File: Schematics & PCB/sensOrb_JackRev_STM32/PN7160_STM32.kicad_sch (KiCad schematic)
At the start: 3 parts, among them J1 USB_C_Receptacle_USB2.0_16P, U1 PN7160A1HN/C100E, U2 STM32F411CEUx

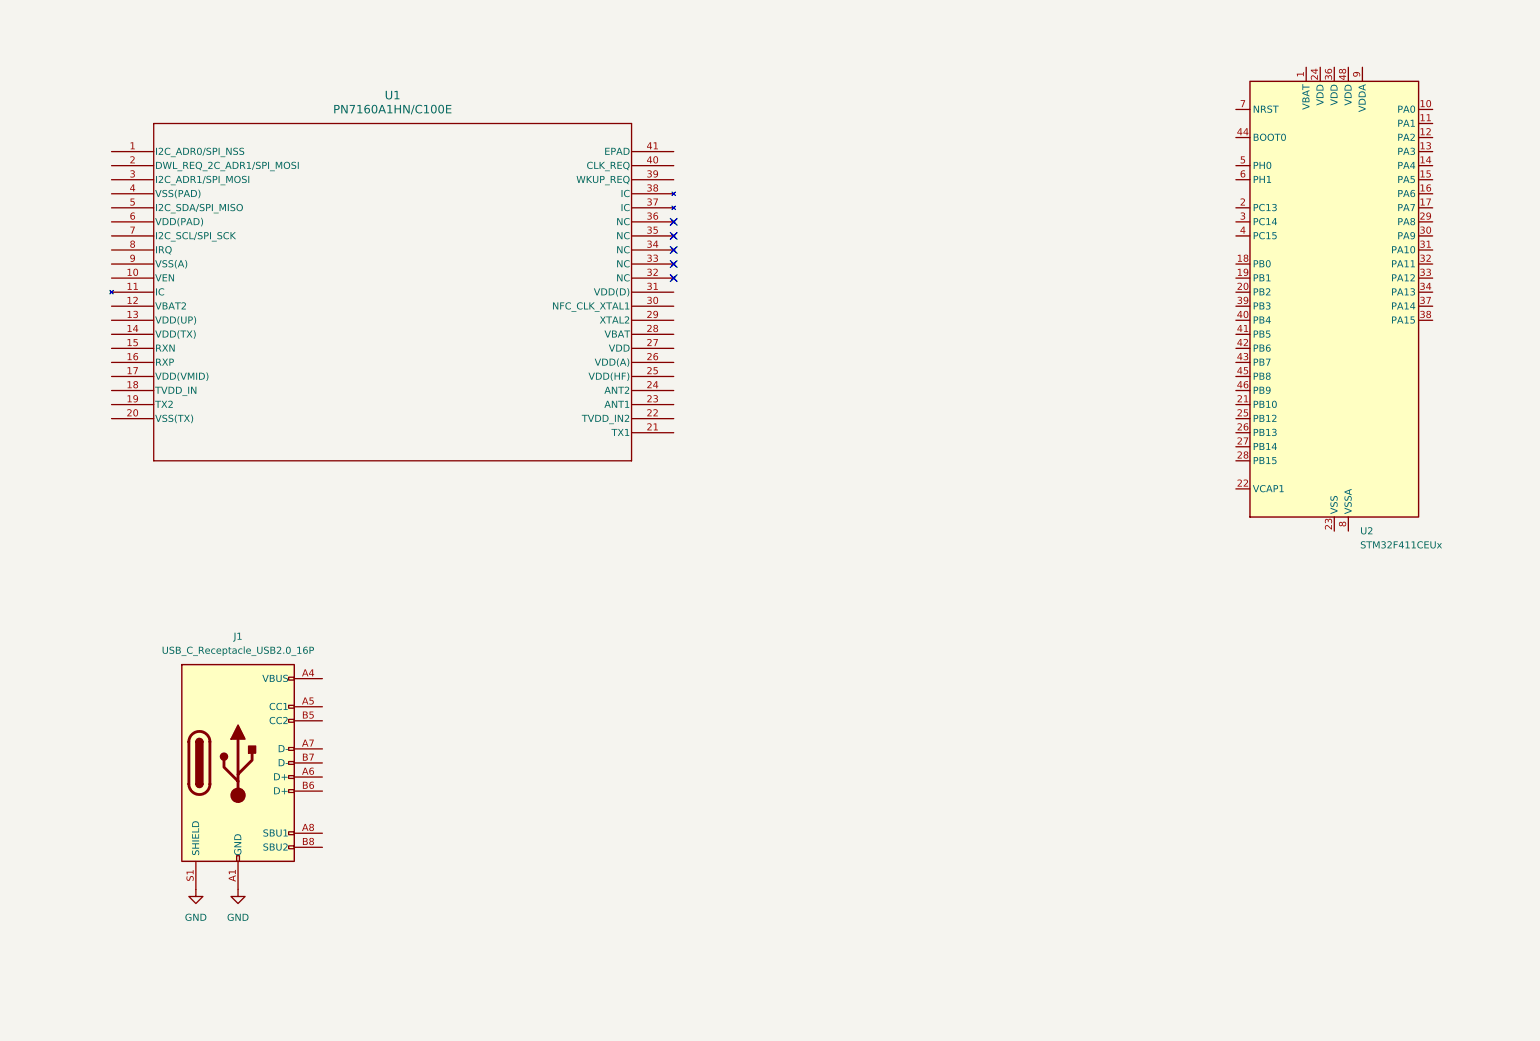
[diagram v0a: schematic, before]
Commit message: Baro unit design complete, core unit nearly done
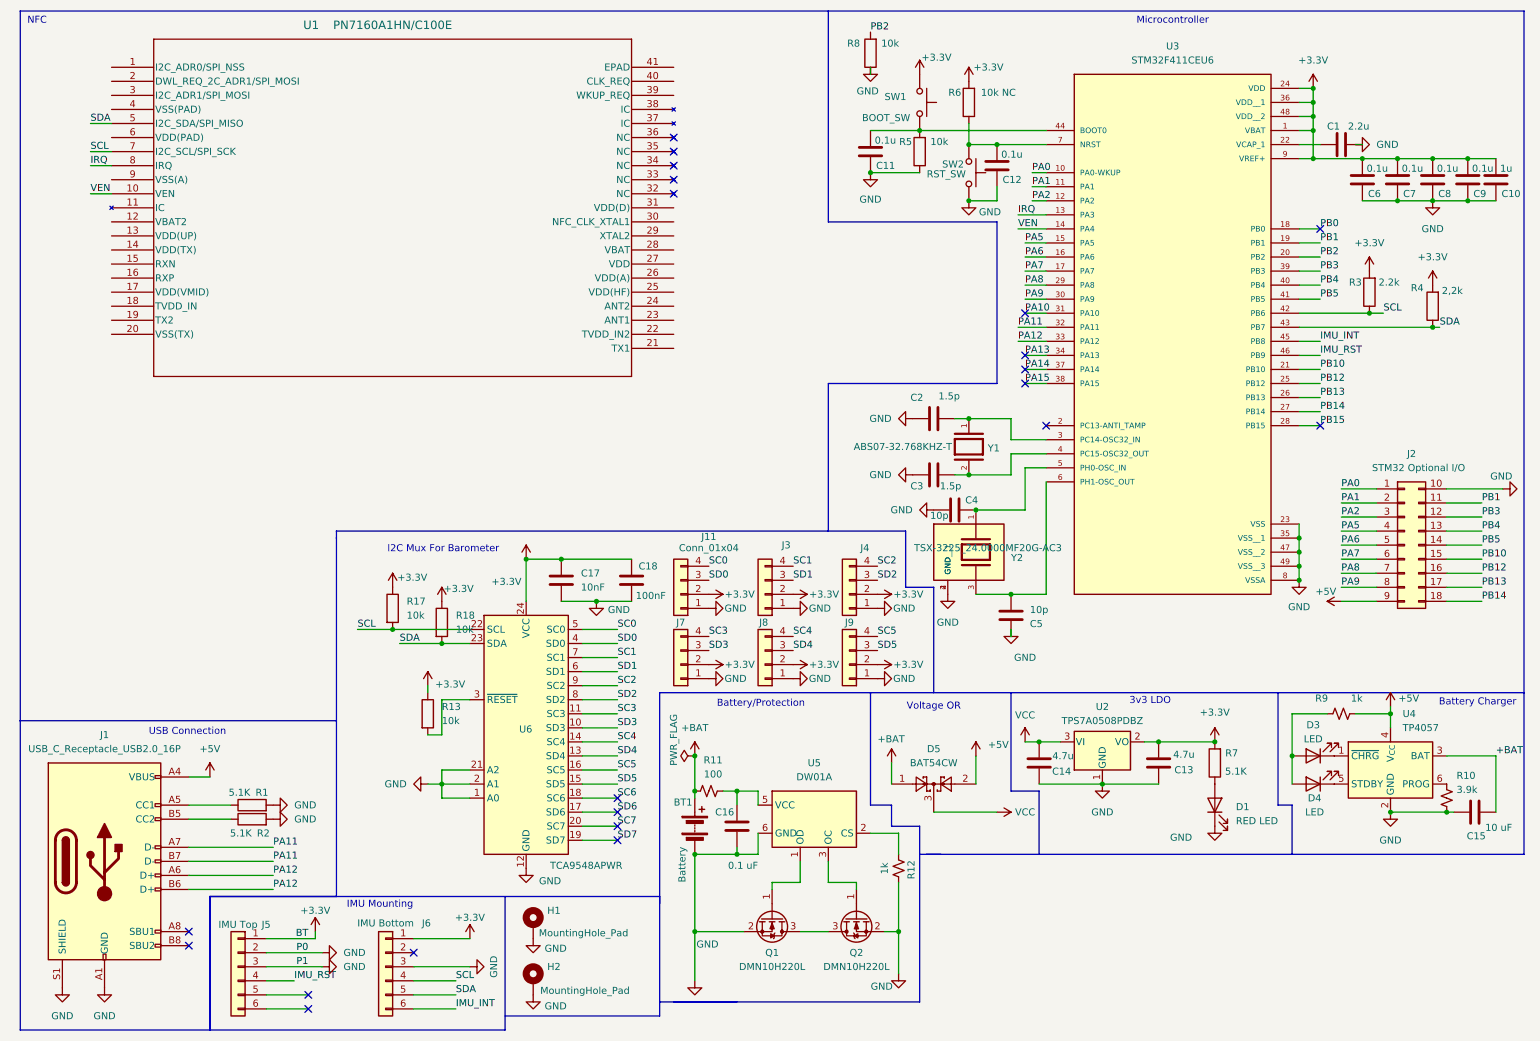
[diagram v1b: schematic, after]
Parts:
- removed U2: STM32F411CEUx, Package_DFN_QFN:QFN-48-1EP_7x7mm_P0.5mm_EP5.6x5.6mm, symbol MCU_ST_STM32F4:STM32F411CEUx
- added BT1: Battery, Battery:BatteryHolder_Keystone_1060_1x2032, symbol Device:Battery
- added C1: 2.2u, symbol Device:C
- added C10: 1u, symbol Device:C
- added C11, C12, C6, C7, C8, C9: 0.1u, symbol Device:C
- added C13, C14: 4.7u, symbol Device:C
- added C15: 10 uF, Capacitor_SMD:C_0805_2012Metric_Pad1.18x1.45mm_HandSolder, symbol Device:C
- added C16: 0.1 uF, Capacitor_SMD:C_0805_2012Metric_Pad1.18x1.45mm_HandSolder, symbol Device:C
- added C17: 10nF, Capacitor_SMD:C_0805_2012Metric_Pad1.18x1.45mm_HandSolder, symbol Device:C
- added C18: 100nF, Capacitor_SMD:C_0805_2012Metric_Pad1.18x1.45mm_HandSolder, symbol Device:C
- added C2, C3: 1.5p, symbol Device:C
- added C4, C5: 10p, symbol Device:C
- added D1: RED LED, symbol Device:LED
- added D3, D4: LED, LED_SMD:LED_0805_2012Metric, symbol Device:LED
- added D5: BAT54CW, Package_TO_SOT_SMD:SOT-323_SC-70, symbol Diode:BAT54CW
- added H1, H2: MountingHole_Pad, MountingHole:MountingHole_2.2mm_M2_Pad, symbol Mechanical:MountingHole_Pad
- added J11, J3, J4, J7, J8, J9: Conn_01x04, Connector_JST:JST_XH_B4B-XH-AM_1x04_P2.50mm_Vertical, symbol Connector_Generic:Conn_01x04
- added J2: STM32 Optional I/O, Connector_PinSocket_2.54mm:PinSocket_2x09_P2.54mm_Vertical, symbol Connector_Generic:Conn_02x09_Top_Bottom
- added J5: IMU Top, Connector_PinSocket_2.54mm:PinSocket_1x06_P2.54mm_Vertical, symbol Connector_Generic:Conn_01x06
- added J6: IMU Bottom, Connector_PinSocket_2.54mm:PinSocket_1x06_P2.54mm_Vertical, symbol Connector_Generic:Conn_01x06
- added Q1, Q2: DMN10H220L, Package_TO_SOT_SMD:SOT-23, symbol Transistor_FET:DMN10H220L
- added R1, R2, R7: 5.1K, symbol Device:R
- added R10: 3.9k, Resistor_SMD:R_0805_2012Metric_Pad1.20x1.40mm_HandSolder, symbol Device:R_Small_US
- added R11: 100, Resistor_SMD:R_0805_2012Metric_Pad1.20x1.40mm_HandSolder, symbol Device:R_Small_US
- added R12, R9: 1k, Resistor_SMD:R_0805_2012Metric_Pad1.20x1.40mm_HandSolder, symbol Device:R_Small_US
- added R13, R17, R18: 10k, Resistor_SMD:R_0805_2012Metric_Pad1.20x1.40mm_HandSolder, symbol Device:R
- added R3: 2.2k, symbol Device:R
- added R4: 2,2k, symbol Device:R
- added R5, R8: 10k, symbol Device:R
- added R6: 10k NC, symbol Device:R
- added SW1: BOOT_SW, symbol Switch:SW_Push
- added SW2: RST_SW, symbol Switch:SW_Push
- added U2: TPS7A0508PDBZ, Package_TO_SOT_SMD:SOT-23, symbol Regulator_Linear:TPS7A0508PDBZ
- added U3: STM32F411CEU6, footprints:QFN50P700X700X60-49N, symbol STM32F411CEU6:STM32F411CEU6
- added U4: TP4057, Package_TO_SOT_SMD:TSOT-23-6, symbol Battery_Management:TP4057
- added U5: DW01A, Package_TO_SOT_SMD:SOT-23-6, symbol Battery_Management:DW01A
- added U6: TCA9548APWR, Package_SO:TSSOP-24_4.4x7.8mm_P0.65mm, symbol Interface_Expansion:TCA9548APWR
- added Y1: ABS07-32.768KHZ-T, ABS07-32.768KHZ-T:XTAL_ABS07-32.768KHZ-T, symbol ABS07-32.768KHZ-T:ABS07-32.768KHZ-T
- added Y2: TSX-3225_24.0000MF20G-AC3, TSX-3225_24.0000MF20G-AC3:XTAL_TSX-3225_24.0000MF20G-AC3, symbol TSX-3225_24.0000MF20G-AC3:TSX-3225_24.0000MF20G-AC3
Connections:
- net GND: now also BT1.2 (-), C1.2, C10.2, C11.2, C12.2, C13.1, C14.1, C15.1, C16.1, C17.2, C18.2, C2.2, C3.1, C4.2, C5.1, C6.2, C7.2, C8.2, C9.2, D1.1 (K), H1.1, H2.1, J11.1 (Pin_1), J2.10 (Pin_10), J3.1 (Pin_1), J4.1 (Pin_1), J5.2 (Pin_2), J5.3 (Pin_3), J6.3 (Pin_3), J7.1 (Pin_1), J8.1 (Pin_1), J9.1 (Pin_1), Q1.2 (S), Q2.2 (S), R1.2, R10.1, R12.1, R2.2, R5.1, R8.1, SW2.2, U2.1 (GND), U3.23 (VSS), U3.35 (VSS__1), U3.47 (VSS__2), U3.49 (VSS__3), U3.8 (VSSA), U4.2 (GND), U5.6 (GND), U6.1 (A0), U6.12 (GND), U6.2 (A1), U6.21 (A2), Y2.2 (GND), Y2.4 (GND__1)
- net +5V: now reaches J1.A4 (VBUS), J1.A9 (VBUS), J1.B4 (VBUS), J1.B9 (VBUS)
- net +5V: now also D5.2, J2.9 (Pin_9), R9.2, U4.4 (V_{CC})
- net at J1.A5 (CC1): now also R1.1
- net PA12: now reaches J1.A6 (D+)
- net PA12: now also J1.B6 (D+), U3.33 (PA12)
- net PA11: now reaches J1.A7 (D-)
- net PA11: now also J1.B7 (D-), U3.32 (PA11)
- net at J1.B5 (CC2): now also R2.1
- net VEN: now reaches U1.10 (VEN)
- net VEN: now also U3.14 (PA4)
- net SDA: now reaches U1.5 (I2C_SDA/SPI_MISO)
- net SDA: now also J6.5 (Pin_5), R18.2, R4.1, U3.43 (PB7), U6.23 (SDA)
- net SCL: now reaches U1.7 (I2C_SCL/SPI_SCK)
- net SCL: now also J6.4 (Pin_4), R17.2, R3.1, U3.42 (PB6), U6.22 (SCL)
- net IRQ: now reaches U1.8 (IRQ)
- net IRQ: now also U3.13 (PA3)
- new net: D4.1 (K), U4.5 (STDBY)
- new net: D3.2 (A), D4.2 (A), R9.1
- new net: C11.1, R5.2, SW1.2, U3.44 (BOOT0)
- new net: Q1.1 (G), U5.1 (OD)
- new net: Q1.3 (D), Q2.3 (D)
- new net: C1.1, U3.22 (VCAP_1)
- new net: C2.1, U3.3 (PC14-OSC32_IN), Y1.1
- new net: C3.2, U3.4 (PC15-OSC32_OUT), Y1.2
- new net: C4.1, U3.5 (PH0-OSC_IN), Y2.1
- new net: C5.2, U3.6 (PH1-OSC_OUT), Y2.3
- new net: C12.1, R6.1, SW2.1, U3.7 (NRST)
- new net: D1.2 (A), R7.1
- new net: Q2.1 (G), U5.3 (OC)
- new net: C16.2, R11.2, U5.5 (VCC)
- new net: D3.1 (K), U4.1 (~{CHRG})
- new net: R10.2, U4.6 (PROG)
- new net: R13.2, U6.3 (~{RESET})
- new net: R12.2, U5.2 (CS)
- new net +3.3V: C10.1, C13.2, C17.1, C18.1, C6.1, C7.1, C8.1, C9.1, J11.2 (Pin_2), J3.2 (Pin_2), J4.2 (Pin_2), J5.1 (Pin_1), J6.1 (Pin_1), J7.2 (Pin_2), J8.2 (Pin_2), J9.2 (Pin_2), R13.1, R17.1, R18.1, R3.2, R4.2, R6.2, R7.2, SW1.1, U2.2 (VO), U3.1 (VBAT), U3.24 (VDD), U3.36 (VDD__1), U3.48 (VDD__2), U3.9 (VREF+), U6.24 (VCC)
- new net +BAT: BT1.1 (+), C15.2, D5.1, R11.1, U4.3 (BAT)
- new net IMU_INT: J6.6 (Pin_6), U3.45 (PB8)
- new net IMU_RST: J5.4 (Pin_4), U3.46 (PB9)
- new net PA0: J2.1 (Pin_1), U3.10 (PA0-WKUP)
- new net PA1: J2.2 (Pin_2), U3.11 (PA1)
- new net PA10: U3.31 (PA10)
- new net PA13: U3.34 (PA13)
- new net PA14: U3.37 (PA14)
- new net PA15: U3.38 (PA15)
- new net PA2: J2.3 (Pin_3), U3.12 (PA2)
- new net PA5: J2.4 (Pin_4), U3.15 (PA5)
- new net PA6: J2.5 (Pin_5), U3.16 (PA6)
- new net PA7: J2.6 (Pin_6), U3.17 (PA7)
- new net PA8: J2.7 (Pin_7), U3.29 (PA8)
- new net PA9: J2.8 (Pin_8), U3.30 (PA9)
- new net PB0: U3.18 (PB0)
- new net PB1: J2.11 (Pin_11), U3.19 (PB1)
- new net PB10: J2.15 (Pin_15), U3.21 (PB10)
- new net PB12: J2.16 (Pin_16), U3.25 (PB12)
- new net PB13: J2.17 (Pin_17), U3.26 (PB13)
- new net PB14: J2.18 (Pin_18), U3.27 (PB14)
- new net PB15: U3.28 (PB15)
- new net PB2: R8.2, U3.20 (PB2)
- new net PB3: J2.12 (Pin_12), U3.39 (PB3)
- new net PB4: J2.13 (Pin_13), U3.40 (PB4)
- new net PB5: J2.14 (Pin_14), U3.41 (PB5)
- new net SC0: J11.4 (Pin_4), U6.5 (SC0)
- new net SC1: J3.4 (Pin_4), U6.7 (SC1)
- new net SC2: J4.4 (Pin_4), U6.9 (SC2)
- new net SC3: J7.4 (Pin_4), U6.11 (SC3)
- new net SC4: J8.4 (Pin_4), U6.14 (SC4)
- new net SC5: J9.4 (Pin_4), U6.16 (SC5)
- new net SC6: U6.18 (SC6)
- new net SC7: U6.20 (SC7)
- new net SD0: J11.3 (Pin_3), U6.4 (SD0)
- new net SD1: J3.3 (Pin_3), U6.6 (SD1)
- new net SD2: J4.3 (Pin_3), U6.8 (SD2)
- new net SD3: J7.3 (Pin_3), U6.10 (SD3)
- new net SD4: J8.3 (Pin_3), U6.13 (SD4)
- new net SD5: J9.3 (Pin_3), U6.15 (SD5)
- new net SD6: U6.17 (SD6)
- new net SD7: U6.19 (SD7)
- new net VCC: C14.2, D5.3, U2.3 (VI)
- no-connect marks 5 -> 21
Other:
- note added: "3v3 LDO"
- note added: "Battery Charger"
- note added: "Battery/Protection"
- note added: "I2C Mux For Barometer"
- note added: "IMU Mounting"
- note added: "Microcontroller"
- note added: "NFC"
- note added: "USB Connection"
- note added: "Voltage OR"
- moved on the sheet: J1, U1
